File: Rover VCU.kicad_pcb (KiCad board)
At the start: 4 copper layers, 86 x 39 mm, 82 parts, among them J1 Conn_ST_STDC14, J2 USB4105-GF-A, J3 430450400, J6 430451200, SW1 TS-1088-AR02016, U1 STM32H563RITx, U3 DP83TC812RRHARQ1, U4 SN65HVD230, U5 SN65HVD230, U6 LMR51610, U7 NXE2S0505MC, U8 NCP1117-3.3_SOT223, Y1 32.768kHz

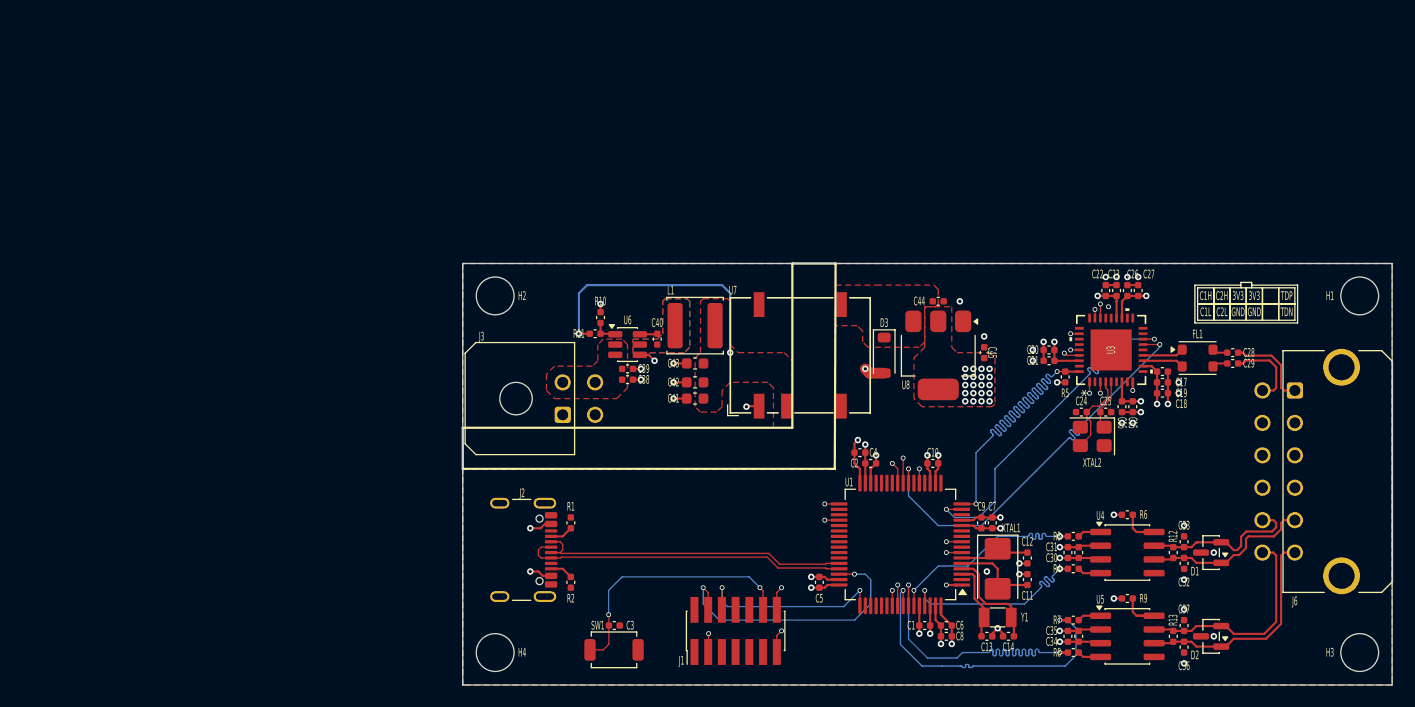
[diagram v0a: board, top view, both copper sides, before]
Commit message: fix: centering board on layout
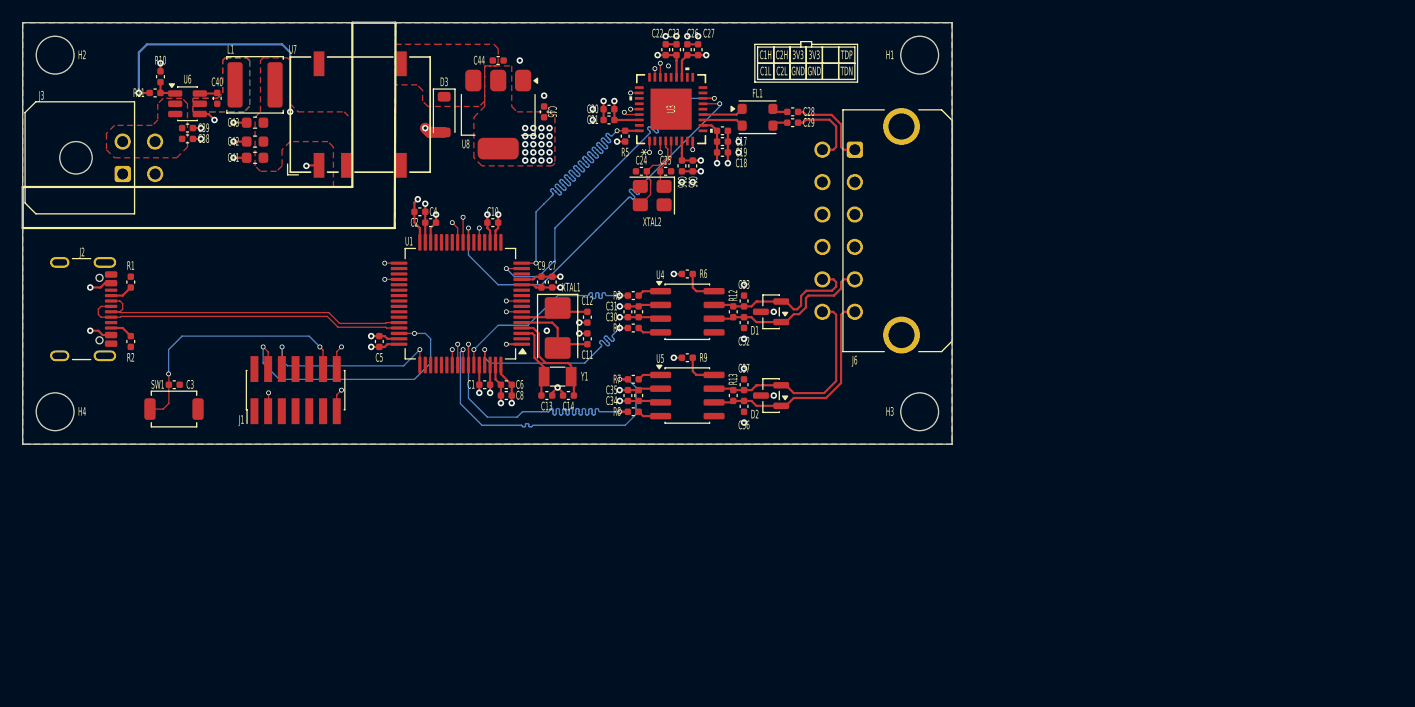
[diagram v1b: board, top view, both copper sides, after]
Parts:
- moved C1 46.4 mm to (142.0, 106.2)
- moved C10 46.4 mm to (142.8, 91.2)
- moved C11 46.4 mm to (151.5, 102.0)
- moved C13 46.4 mm to (147.8, 107.2)
- moved C15 46.4 mm to (161.3, 86.0)
- moved C16 46.4 mm to (160.3, 86.0)
- moved C2 46.4 mm to (137.0, 91.2)
- moved C20 46.4 mm to (153.5, 80.7)
- moved C21 46.4 mm to (153.5, 81.7)
- moved C22 46.4 mm to (158.8, 75.2)
- moved C23 46.4 mm to (159.8, 75.2)
- moved C24 46.4 mm to (156.5, 86.5)
- moved C25 46.4 mm to (158.8, 86.5)
- moved C26 46.4 mm to (160.8, 75.2)
- moved C27 46.4 mm to (161.8, 75.2)
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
